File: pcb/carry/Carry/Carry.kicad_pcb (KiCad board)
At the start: 2 copper layers, 36.3 x 62.5 mm, 3 parts, among them U1 Luckfox-Pico_Mini_B, U2 MCP73831-2-OT

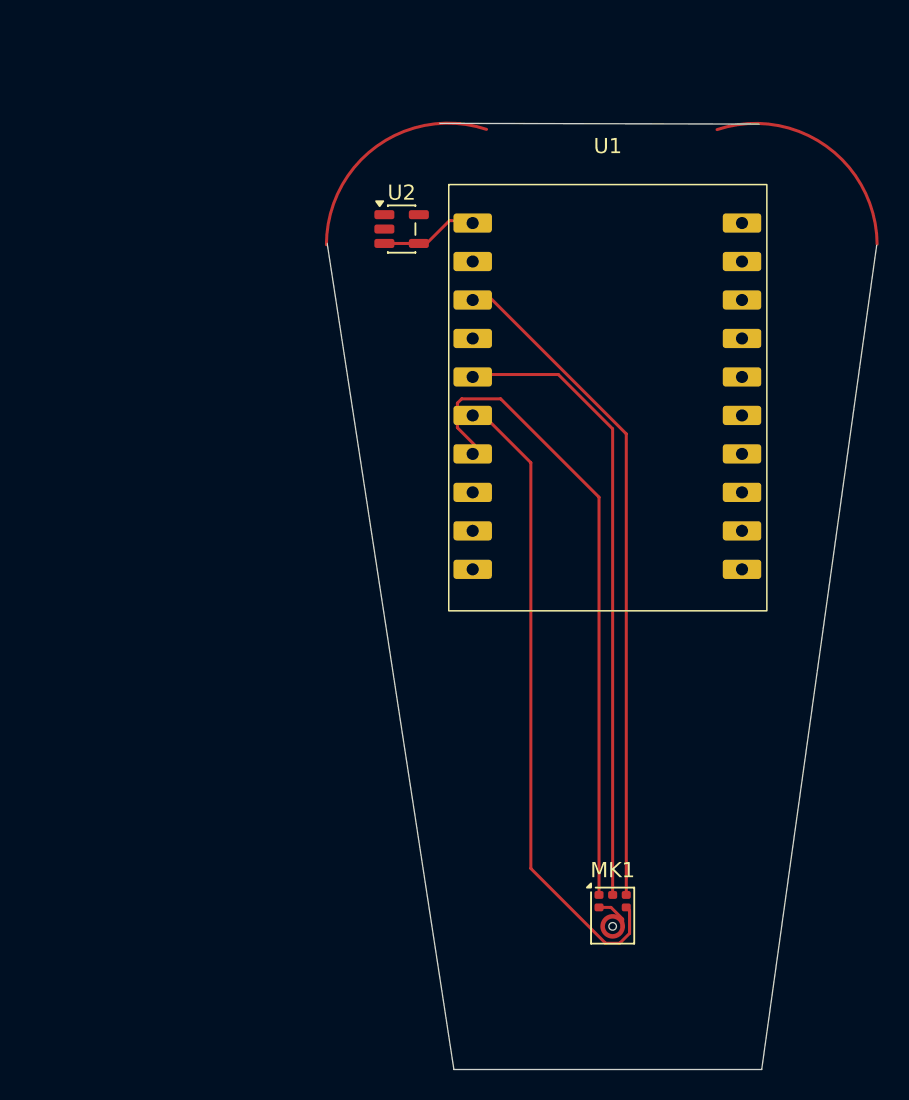
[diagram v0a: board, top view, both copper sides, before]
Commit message: updated
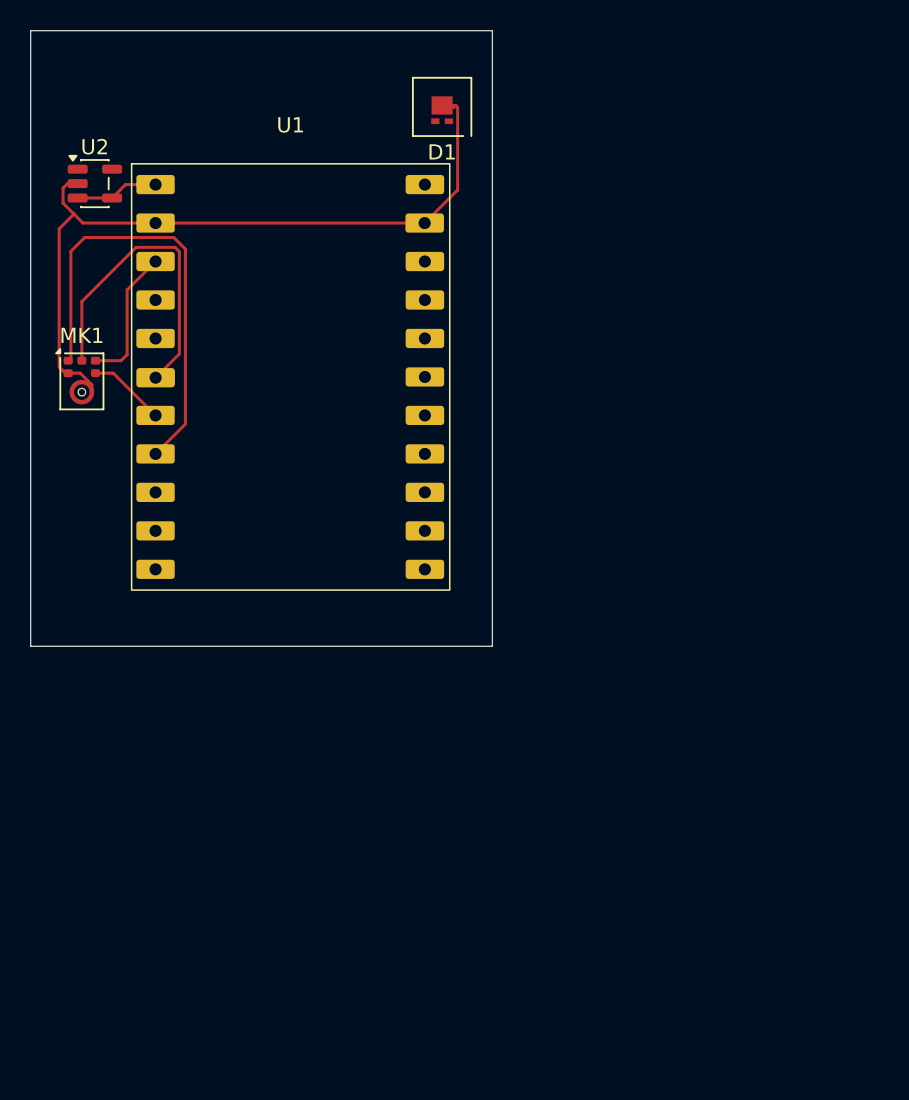
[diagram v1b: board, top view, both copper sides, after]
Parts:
- added D1: LED_Dual_AAK, LED_SMD:LED-L1T2_LUMILEDS, F.Cu at (121.1, 66.4)
- moved MK1 49.7 mm to (97.4, 84.1)
- moved U1 21.0 mm to (111.1, 83.8)
- moved U2 20.5 mm to (98.2, 71.1)
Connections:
- U1 pad 2: unconnected-(U1-GND-Pad2) -> GND
- U1 pad 20: unconnected-(U1-GPIO4_C1_z-Pad20) -> Net-(U1-GPIO4_C1_z)
- U1 pad 21: unconnected-(U1-GND-Pad21) -> GND
- U2 pad 2: unconnected-(U2-V_{SS}-Pad2) -> GND
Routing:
- net GND: track 2.36 -> 50.8 mm
- net Net-(MK1-BCLK): track 42.1 -> 5.12 mm
- net Net-(MK1-VDD): track 43.7 -> 9.18 mm
- net /MIC_DATA: track 40.9 -> 20.9 mm
- net Net-(MK1-WS): track 42.3 -> 29.9 mm
- net Net-(J1-Pin_1): track 7.01 -> 5.51 mm
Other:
- board size 36.3 x 62.5 mm -> 30.5 x 40.6 mm
